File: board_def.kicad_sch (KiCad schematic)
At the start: 1 part

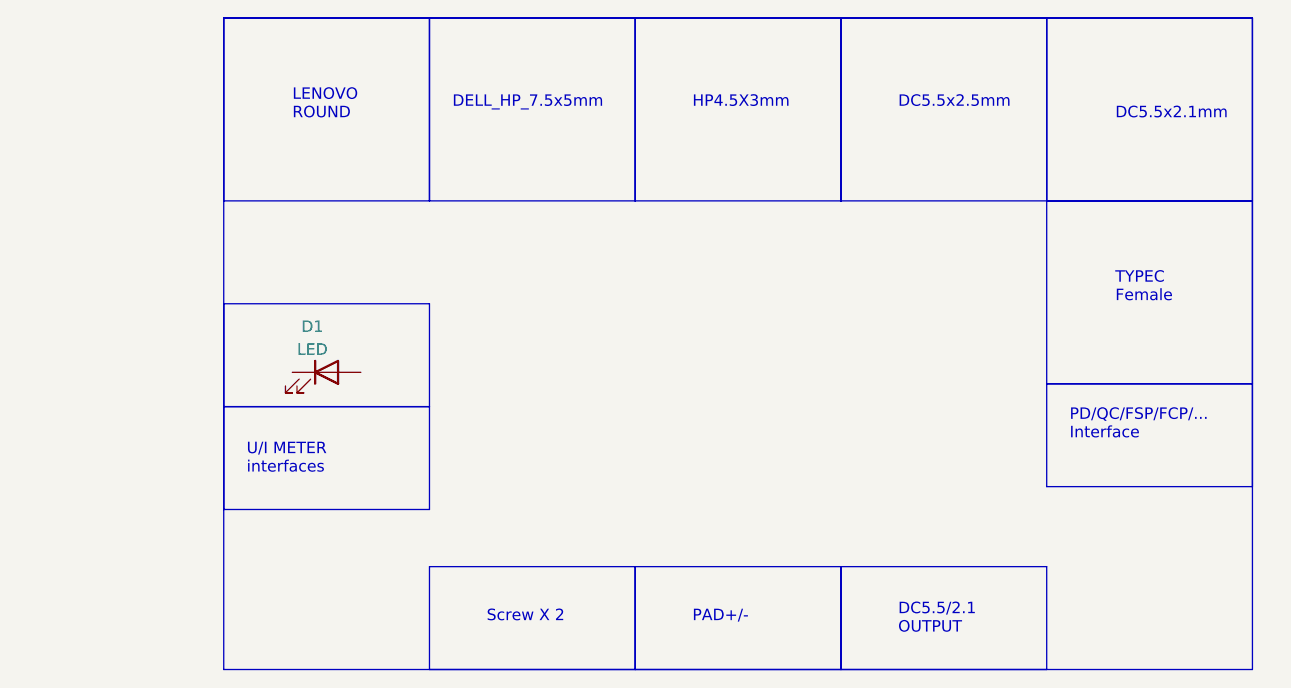
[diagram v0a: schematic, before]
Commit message: more
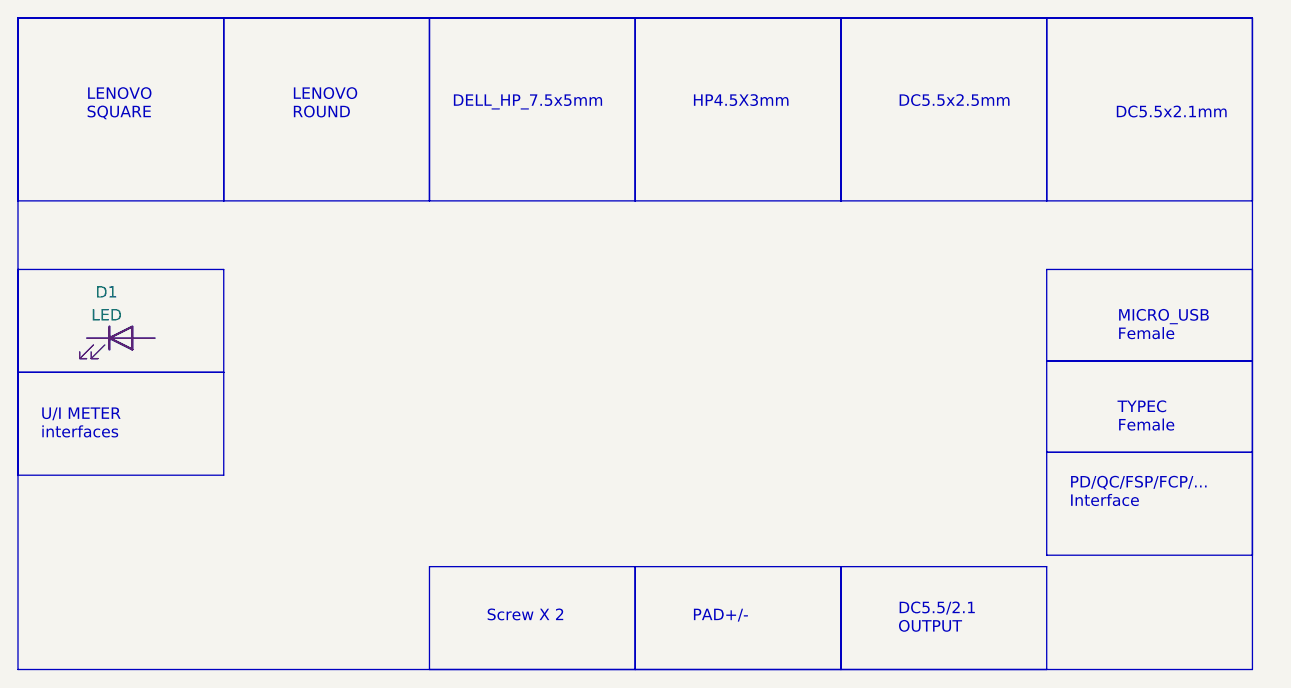
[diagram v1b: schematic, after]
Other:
- note added: "LENOVO SQUARE"
- note added: "MICRO_USB Female"
- moved on the sheet: D1
